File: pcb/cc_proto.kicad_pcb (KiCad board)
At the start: 2 copper layers, 96 x 79 mm, 46 parts, among them SW1 SW_PUSH, SW10 SW_PUSH, SW11 SW_PUSH, SW12 SW_PUSH, SW13 SW_PUSH, SW14 SW_PUSH, SW15 SW_PUSH, SW16 SW_PUSH, SW17 SW_PUSH, SW18 SW_PUSH, SW2 SW_PUSH, SW3 SW_PUSH, SW4 SW_PUSH, SW5 SW_PUSH, SW6 SW_PUSH, SW7 SW_PUSH, SW8 SW_PUSH, SW9 SW_PUSH, U1 ProMicro

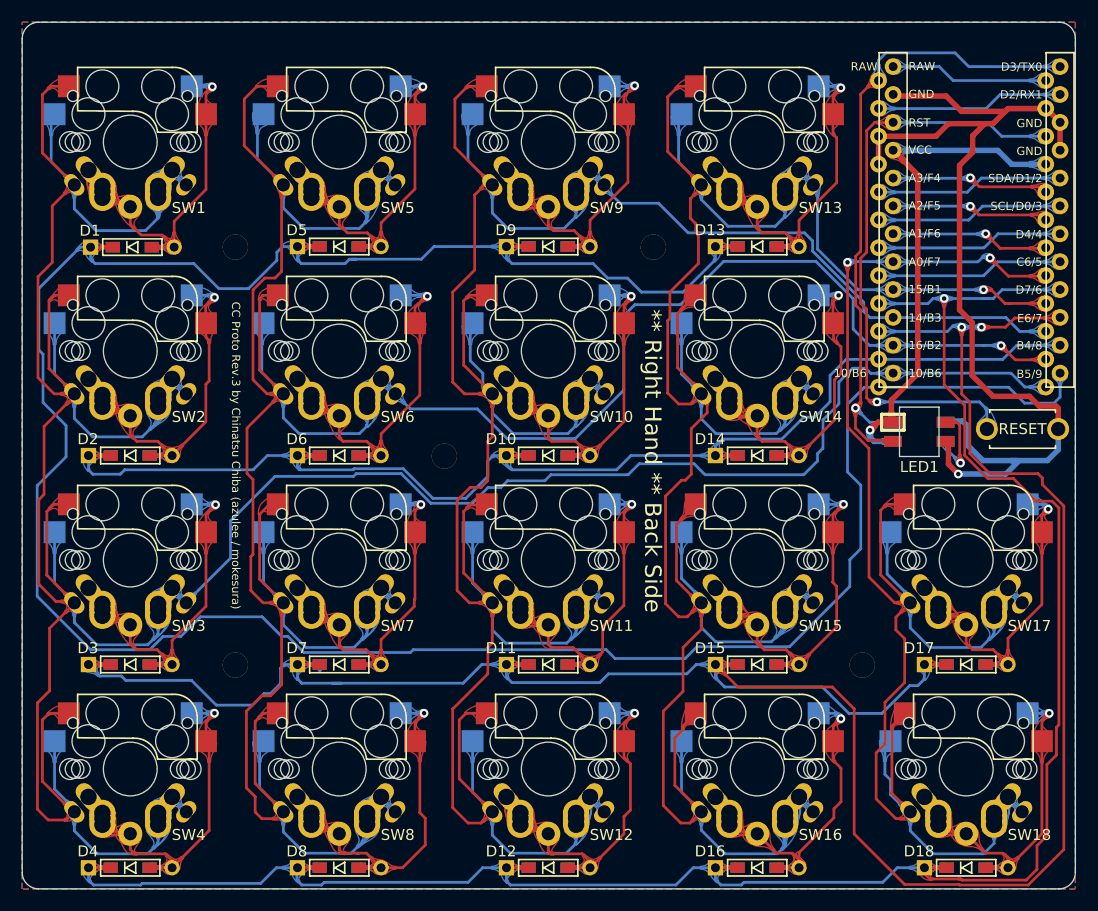
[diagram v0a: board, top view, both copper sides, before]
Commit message: PCB Rev.4
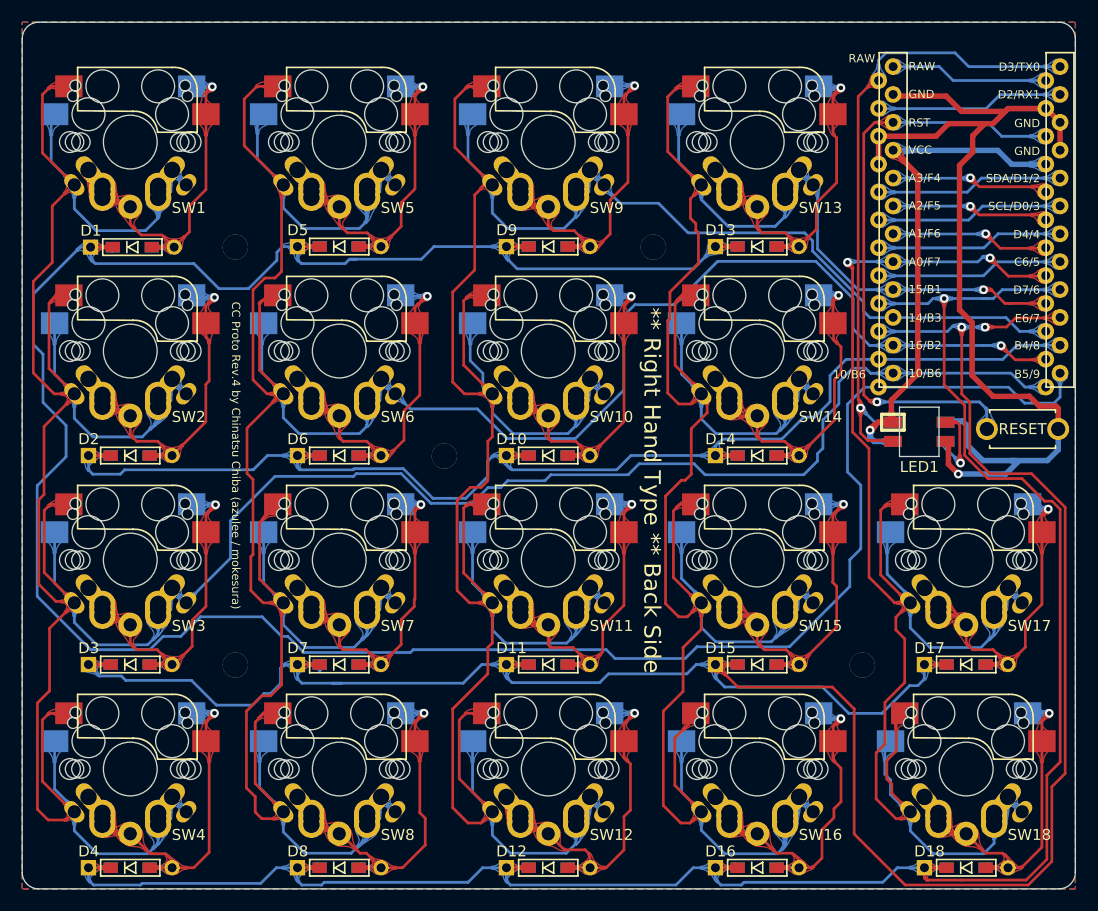
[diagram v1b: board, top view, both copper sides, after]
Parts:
- D1, D10, D11, D12, D13, D14, D15, D16, D17, D18, D2, D3, D4, D5, D6, D7, D8, D9: footprint mokesura_kbd_footprint:D3_TH_SMD -> cc_proto:D3_TH_SMD_Text-Added
- LED1: footprint mokesura_kbd_footprint:SK6812MINI_rev -> cc_proto:SK6812MINI_rev_Text-Added
- SW1, SW10, SW11, SW12, SW13, SW14, SW15, SW16, SW17, SW18, SW2, SW3, SW4, SW5, SW6, SW7, SW8, SW9: footprint mokesura_kbd_footprint:CherryMX_MidHeight_Hotswap_Choc_Alps_v2 -> cc_proto:CherryMX_MidHeight_Hotswap_Choc12_Alps_v2
- U1: footprint mokesura_kbd_footprint:ProMicro_v2 -> cc_proto:ProMicro_v2_Text-Changed
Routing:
- net Row0: track 245.1 -> 243.1 mm
- net Net-(D8-Pad2): track 35.3 -> 33.4 mm
- net Col1: track 290.1 -> 288.6 mm
- net Col3: track 244.4 -> 245.6 mm
- net LED: track 60.4 -> 59.4 mm
- net Col2: track 266.2 -> 265.5 mm
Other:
- board text added: "** Right Hand Type ** Back Side"
- board text added: "++ Left Hand Type ++ Back Side"
- board text added: "CC Proto Rev.4 by Chinatsu Chiba (azulee / mokesura)"
- board text removed: "** Right Hand ** Back Side"
- board text removed: "++ Left Hand ++ Back Side"
- board text removed: "CC Proto Rev.3 by Chinatsu Chiba (azulee / mokesura)"
